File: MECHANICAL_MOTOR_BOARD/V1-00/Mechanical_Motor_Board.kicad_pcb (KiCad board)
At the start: 2 copper layers, 88.9 x 44.5 mm, 83 parts, among them K1 COLONETTE, K2 COLONETTE, K3 COLONETTE, K4 COLONETTE, P1001 CONN_02X13, P1002 CONN_02X08, P1003 CONN_01X02, P1004 CONN_01X02, P1005 CONN_01X04, P1006 CONN_01X04, Q2001 2N7002, Q3003 BSR14, Q3004 BSR14, Q3005 BTS50055, Q3006 BTS50055, Q3007 STB80NF55L_06T4, Q3008 STB80NF55L_06T4, Q3009 STB80NF55L_06T4, Q3010 STB80NF55L_06T4, Q3011 BTS50055, Q3012 BTS50055, Q3013 BSR14, Q3014 BSR14, U2001 HCTL-2032, U2002 M74VHC1GT02DTT1G, U3001 74HC02, U3002 74HC02, X2001 12Mhz

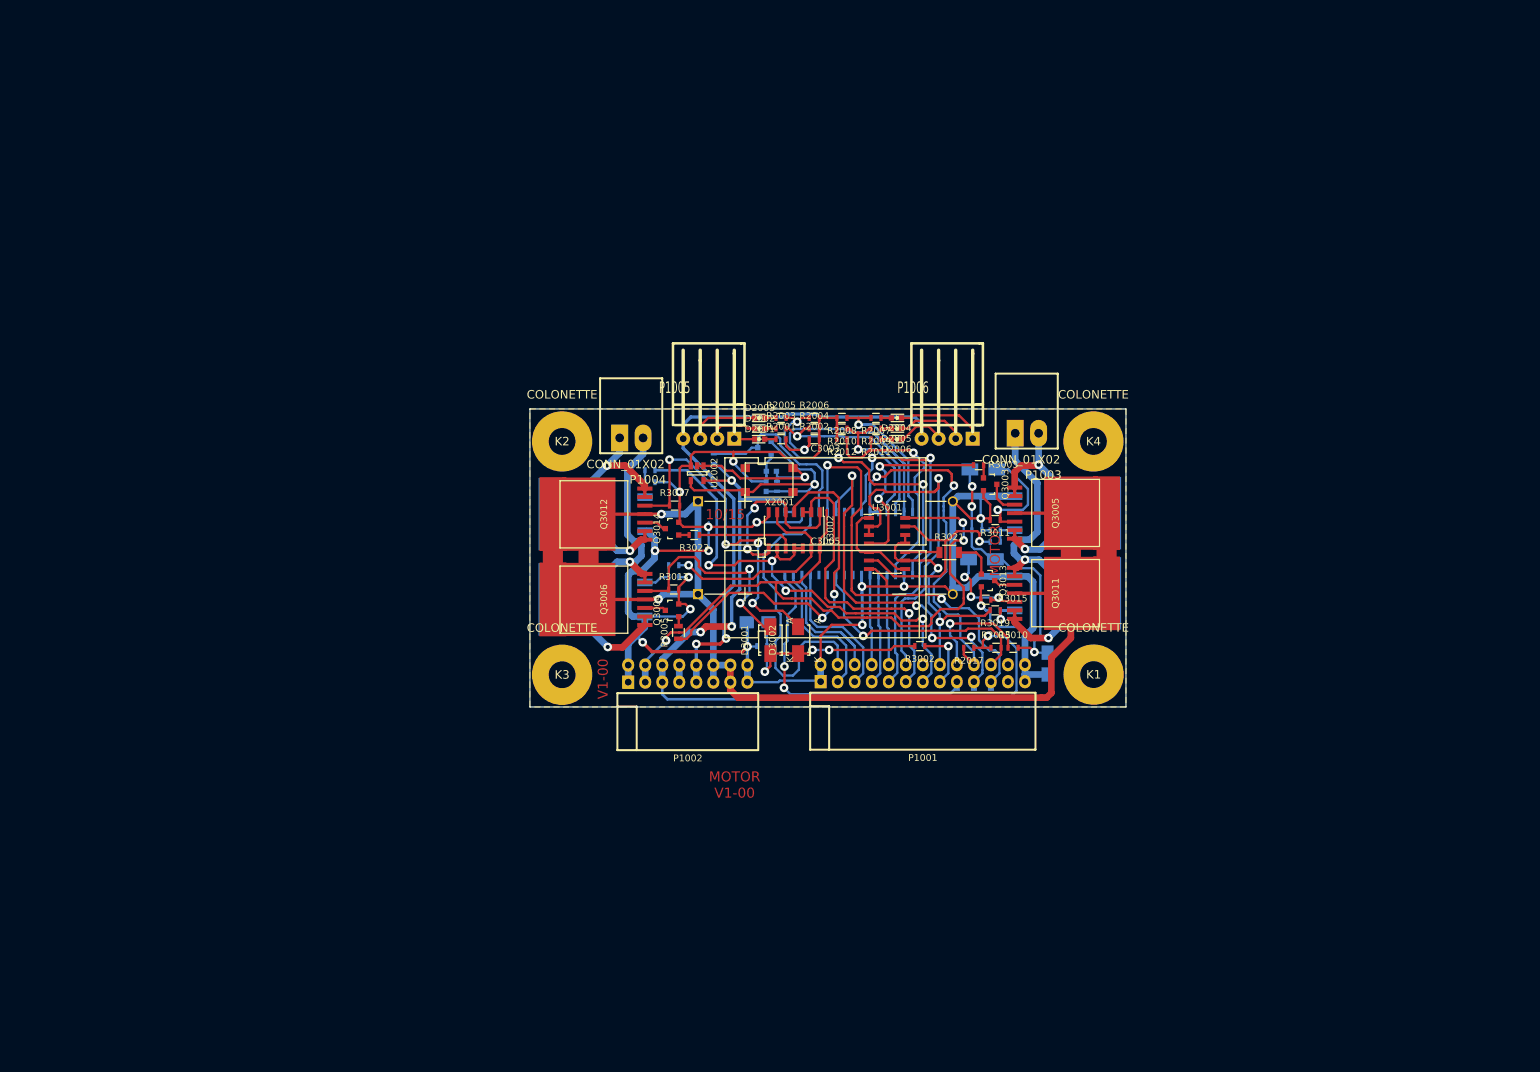
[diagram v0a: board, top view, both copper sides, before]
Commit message: MAJ 2018
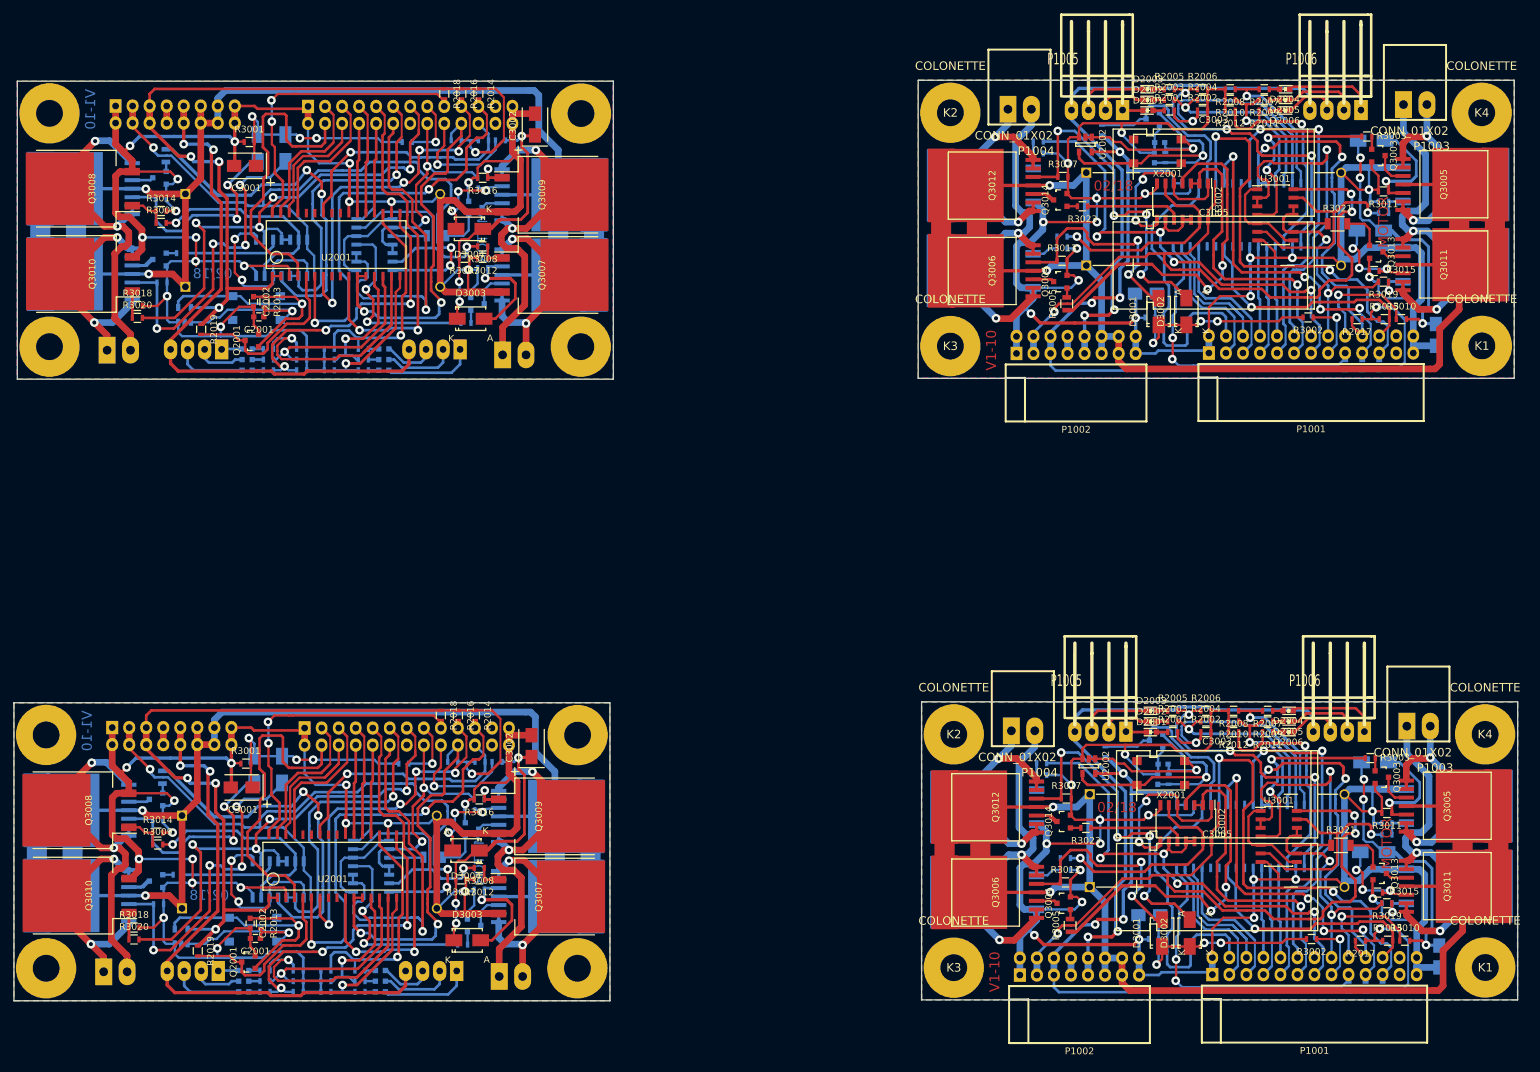
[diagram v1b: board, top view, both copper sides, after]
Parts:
- added C2001: 27p, Capacitors_SMD:C_0603, F.Cu at (73.3, 164.6)
- added C2001: 27p, Capacitors_SMD:C_0603, F.Cu at (73.8, 71.9)
- added C2001: 27p, Capacitors_SMD:C_0603, B.Cu at (208.7, 138.6)
- added C2002: 27p, Capacitors_SMD:C_0603, F.Cu at (72.5, 162.4)
- added C2002: 27p, Capacitors_SMD:C_0603, F.Cu at (73.0, 69.7)
- added C2002: 27p, Capacitors_SMD:C_0603, B.Cu at (207.9, 140.9)
- added C3001: 10u, Capacitors_Tantalum_SMD:TantalC_SizeB_EIA-3528_Wave, F.Cu at (71.2, 142.1)
- added C3001: 10u, Capacitors_Tantalum_SMD:TantalC_SizeB_EIA-3528_Wave, F.Cu at (71.8, 49.4)
- added C3001: 10u, Capacitors_Tantalum_SMD:TantalC_SizeB_EIA-3528_Wave, B.Cu at (206.6, 161.2)
- added C3002: 10u, Capacitors_Tantalum_SMD:TantalC_SizeB_EIA-3528_Wave, F.Cu at (114.5, 136.0)
- added C3002: 10u, Capacitors_Tantalum_SMD:TantalC_SizeB_EIA-3528_Wave, F.Cu at (115.0, 43.2)
- added C3002: 10u, Capacitors_Tantalum_SMD:TantalC_SizeB_EIA-3528_Wave, B.Cu at (249.9, 167.3)
- added C3003: 470U, Capacitors_ThroughHole:C_Axial_D13_L31_P38, B.Cu at (62.4, 160.1)
- added C3003: 470U, Capacitors_ThroughHole:C_Axial_D13_L31_P38, B.Cu at (62.9, 67.4)
- added C3003: 470U, Capacitors_ThroughHole:C_Axial_D13_L31_P38, F.Cu at (197.7, 143.1)
- added C3005: CP, Capacitors_ThroughHole:C_Axial_D13_L31_P38, B.Cu at (62.4, 146.3)
- added C3005: CP, Capacitors_ThroughHole:C_Axial_D13_L31_P38, B.Cu at (62.9, 53.6)
- added C3005: CP, Capacitors_ThroughHole:C_Axial_D13_L31_P38, F.Cu at (197.7, 157.0)
- added D2001: LED, LEDs:LED-0603, B.Cu at (71.6, 169.4)
- added D2001: LED, LEDs:LED-0603, B.Cu at (72.1, 76.7)
- added D2001: LED, LEDs:LED-0603, F.Cu at (206.9, 133.9)
- added D2002: LED, LEDs:LED-0603, B.Cu at (71.6, 171.0)
- added D2002: LED, LEDs:LED-0603, B.Cu at (72.1, 78.3)
- added D2002: LED, LEDs:LED-0603, F.Cu at (206.9, 132.3)
- added D2003: LED, LEDs:LED-0603, B.Cu at (71.6, 172.6)
- added D2003: LED, LEDs:LED-0603, B.Cu at (72.1, 79.9)
- added D2003: LED, LEDs:LED-0603, F.Cu at (206.9, 130.7)
- added D2004: LED, LEDs:LED-0603, B.Cu at (91.9, 172.6)
- added D2004: LED, LEDs:LED-0603, B.Cu at (92.5, 79.9)
- added D2004: LED, LEDs:LED-0603, F.Cu at (227.3, 130.7)
- added D2005: LED, LEDs:LED-0603, B.Cu at (91.9, 171.0)
- added D2005: LED, LEDs:LED-0603, B.Cu at (92.5, 78.3)
- added D2005: LED, LEDs:LED-0603, F.Cu at (227.3, 132.3)
- added D2006: LED, LEDs:LED-0603, B.Cu at (91.9, 169.4)
- added D2006: LED, LEDs:LED-0603, B.Cu at (92.5, 76.7)
- added D2006: LED, LEDs:LED-0603, F.Cu at (227.3, 133.9)
- added D3001: B140, Diodes_SMD:Diode-SMA_Standard, B.Cu at (73.2, 139.4)
- added D3001: B140, Diodes_SMD:Diode-SMA_Standard, B.Cu at (73.7, 46.7)
- added D3001: B140, Diodes_SMD:Diode-SMA_Standard, F.Cu at (208.5, 163.8)
- added D3002: B140, Diodes_SMD:Diode-SMA_Standard, B.Cu at (77.3, 139.4)
- added D3002: B140, Diodes_SMD:Diode-SMA_Standard, B.Cu at (77.8, 46.7)
- added D3002: B140, Diodes_SMD:Diode-SMA_Standard, F.Cu at (212.7, 163.8)
- added D3003: B140, Diodes_SMD:Diode-SMA_Standard, F.Cu at (104.9, 164.9)
- added D3003: B140, Diodes_SMD:Diode-SMA_Standard, F.Cu at (105.4, 72.2)
- added D3003: B140, Diodes_SMD:Diode-SMA_Standard, B.Cu at (240.3, 138.4)
- added D3004: B140, Diodes_SMD:Diode-SMA_Standard, F.Cu at (104.7, 151.5)
- added D3004: B140, Diodes_SMD:Diode-SMA_Standard, F.Cu at (105.2, 58.8)
- added D3004: B140, Diodes_SMD:Diode-SMA_Standard, B.Cu at (240.1, 151.8)
- added K1: COLONETTE, CEN-PCB:COLONETTE, B.Cu at (121.4, 134.3)
- added K1: COLONETTE, CEN-PCB:COLONETTE, B.Cu at (121.9, 41.6)
- added K1: COLONETTE, CEN-PCB:COLONETTE, F.Cu at (256.7, 169.0)
- added K2: COLONETTE, CEN-PCB:COLONETTE, B.Cu at (42.1, 169.1)
- added K2: COLONETTE, CEN-PCB:COLONETTE, B.Cu at (42.6, 76.4)
- added K2: COLONETTE, CEN-PCB:COLONETTE, F.Cu at (177.5, 134.2)
- added K3: COLONETTE, CEN-PCB:COLONETTE, B.Cu at (42.1, 134.3)
- added K3: COLONETTE, CEN-PCB:COLONETTE, B.Cu at (42.6, 41.6)
- added K3: COLONETTE, CEN-PCB:COLONETTE, F.Cu at (177.5, 169.0)
- added K4: COLONETTE, CEN-PCB:COLONETTE, B.Cu at (121.3, 169.1)
- added K4: COLONETTE, CEN-PCB:COLONETTE, B.Cu at (121.8, 76.4)
- added K4: COLONETTE, CEN-PCB:COLONETTE, F.Cu at (256.7, 134.2)
- added P1001: CONN_02X13, w_pin_strip:pin_socket_13x2-90, B.Cu at (95.9, 129.6)
- added P1001: CONN_02X13, w_pin_strip:pin_socket_13x2-90, B.Cu at (96.4, 36.9)
- added P1001: CONN_02X13, w_pin_strip:pin_socket_13x2-90, F.Cu at (231.3, 173.7)
- added P1002: CONN_02X08, w_pin_strip:pin_socket_8x2-90, B.Cu at (60.8, 129.5)
- added P1002: CONN_02X08, w_pin_strip:pin_socket_8x2-90, B.Cu at (61.3, 36.8)
- added P1002: CONN_02X08, w_pin_strip:pin_socket_8x2-90, F.Cu at (196.2, 173.7)
- added P1003: CONN_01X02, CEN-PCB:WEIDMULLER-SL-3.5-2-90G, B.Cu at (109.7, 170.3)
- added P1003: CONN_01X02, CEN-PCB:WEIDMULLER-SL-3.5-2-90G, B.Cu at (110.2, 77.6)
- added P1003: CONN_01X02, CEN-PCB:WEIDMULLER-SL-3.5-2-90G, F.Cu at (245.0, 133.0)
- added P1004: CONN_01X02, CEN-PCB:WEIDMULLER-SL-3.5-2-90G, B.Cu at (50.7, 169.6)
- added P1004: CONN_01X02, CEN-PCB:WEIDMULLER-SL-3.5-2-90G, B.Cu at (51.2, 76.9)
- added P1004: CONN_01X02, CEN-PCB:WEIDMULLER-SL-3.5-2-90G, F.Cu at (186.1, 133.7)
- added P1005: CONN_01X04, CEN-PCB:KK-4-H, B.Cu at (60.1, 169.5)
- added P1005: CONN_01X04, CEN-PCB:KK-4-H, B.Cu at (60.7, 76.8)
- added P1005: CONN_01X04, CEN-PCB:KK-4-H, F.Cu at (195.5, 133.8)
- added P1006: CONN_01X04, CEN-PCB:KK-4-H, B.Cu at (95.7, 169.5)
- added P1006: CONN_01X04, CEN-PCB:KK-4-H, B.Cu at (96.2, 76.8)
- added P1006: CONN_01X04, CEN-PCB:KK-4-H, F.Cu at (231.1, 133.8)
- added Q2001: 2N7002, Housings_SOT-23_SOT-143_TSOT-6:SOT-23, F.Cu at (72.3, 168.1)
- added Q2001: 2N7002, Housings_SOT-23_SOT-143_TSOT-6:SOT-23, F.Cu at (72.8, 75.4)
- added Q2001: 2N7002, Housings_SOT-23_SOT-143_TSOT-6:SOT-23, B.Cu at (207.6, 135.1)
- added Q3003: BSR14, Housings_SOT-23_SOT-143_TSOT-6:SOT-23, B.Cu at (105.9, 162.7)
- added Q3003: BSR14, Housings_SOT-23_SOT-143_TSOT-6:SOT-23, B.Cu at (106.4, 70.0)
- added Q3003: BSR14, Housings_SOT-23_SOT-143_TSOT-6:SOT-23, F.Cu at (241.3, 140.6)
- added Q3004: BSR14, Housings_SOT-23_SOT-143_TSOT-6:SOT-23, B.Cu at (58.5, 143.9)
- added Q3004: BSR14, Housings_SOT-23_SOT-143_TSOT-6:SOT-23, B.Cu at (59.0, 51.2)
- added Q3004: BSR14, Housings_SOT-23_SOT-143_TSOT-6:SOT-23, F.Cu at (193.9, 159.4)
- added Q3005: BTS50055, f4deb-mod-library:PG-TO220-7-4, B.Cu at (109.6, 158.4)
- added Q3005: BTS50055, f4deb-mod-library:PG-TO220-7-4, B.Cu at (110.1, 65.7)
- added Q3005: BTS50055, f4deb-mod-library:PG-TO220-7-4, F.Cu at (245.0, 144.9)
- added Q3006: BTS50055, f4deb-mod-library:PG-TO220-7-4, B.Cu at (54.4, 145.5)
- added Q3006: BTS50055, f4deb-mod-library:PG-TO220-7-4, B.Cu at (54.9, 52.8)
- added Q3006: BTS50055, f4deb-mod-library:PG-TO220-7-4, F.Cu at (189.8, 157.8)
- added Q3007: STB80NF55L_06T4, SMD_Packages:TO-263, F.Cu at (109.6, 158.4)
- added Q3007: STB80NF55L_06T4, SMD_Packages:TO-263, F.Cu at (110.1, 65.7)
- added Q3007: STB80NF55L_06T4, SMD_Packages:TO-263, B.Cu at (245.0, 144.9)
- added Q3008: STB80NF55L_06T4, SMD_Packages:TO-263, F.Cu at (54.4, 145.5)
- added Q3008: STB80NF55L_06T4, SMD_Packages:TO-263, F.Cu at (54.9, 52.8)
- added Q3008: STB80NF55L_06T4, SMD_Packages:TO-263, B.Cu at (189.8, 157.8)
- added Q3009: STB80NF55L_06T4, SMD_Packages:TO-263, F.Cu at (109.6, 146.4)
- added Q3009: STB80NF55L_06T4, SMD_Packages:TO-263, F.Cu at (110.1, 53.7)
- added Q3009: STB80NF55L_06T4, SMD_Packages:TO-263, B.Cu at (245.0, 156.9)
- added Q3010: STB80NF55L_06T4, SMD_Packages:TO-263, F.Cu at (54.4, 158.2)
- added Q3010: STB80NF55L_06T4, SMD_Packages:TO-263, F.Cu at (55.0, 65.5)
- added Q3010: STB80NF55L_06T4, SMD_Packages:TO-263, B.Cu at (189.8, 145.0)
- added Q3011: BTS50055, f4deb-mod-library:PG-TO220-7-4, B.Cu at (109.6, 146.4)
- added Q3011: BTS50055, f4deb-mod-library:PG-TO220-7-4, B.Cu at (110.1, 53.7)
- added Q3011: BTS50055, f4deb-mod-library:PG-TO220-7-4, F.Cu at (245.0, 156.9)
- added Q3012: BTS50055, f4deb-mod-library:PG-TO220-7-4, B.Cu at (54.4, 158.2)
- added Q3012: BTS50055, f4deb-mod-library:PG-TO220-7-4, B.Cu at (54.9, 65.5)
- added Q3012: BTS50055, f4deb-mod-library:PG-TO220-7-4, F.Cu at (189.8, 145.0)
- added Q3013: BSR14, Housings_SOT-23_SOT-143_TSOT-6:SOT-23, B.Cu at (105.6, 148.3)
- added Q3013: BSR14, Housings_SOT-23_SOT-143_TSOT-6:SOT-23, B.Cu at (106.1, 55.6)
- added Q3013: BSR14, Housings_SOT-23_SOT-143_TSOT-6:SOT-23, F.Cu at (241.0, 154.9)
- added Q3014: BSR14, Housings_SOT-23_SOT-143_TSOT-6:SOT-23, B.Cu at (58.5, 156.1)
- added Q3014: BSR14, Housings_SOT-23_SOT-143_TSOT-6:SOT-23, B.Cu at (59.0, 63.4)
- added Q3014: BSR14, Housings_SOT-23_SOT-143_TSOT-6:SOT-23, F.Cu at (193.9, 147.2)
- added R2001: 2.1k, Resistors_SMD:R_0603, B.Cu at (74.7, 169.4)
- added R2001: 2.1k, Resistors_SMD:R_0603, B.Cu at (75.2, 76.7)
- added R2001: 2.1k, Resistors_SMD:R_0603, F.Cu at (210.1, 133.9)
- added R2002: 2.1k, Resistors_SMD:R_0603, B.Cu at (79.7, 169.4)
- added R2002: 2.1k, Resistors_SMD:R_0603, B.Cu at (80.2, 76.7)
- added R2002: 2.1k, Resistors_SMD:R_0603, F.Cu at (215.1, 133.9)
- added R2003: 2.1k, Resistors_SMD:R_0603, B.Cu at (74.7, 171.0)
- added R2003: 2.1k, Resistors_SMD:R_0603, B.Cu at (75.2, 78.3)
- added R2003: 2.1k, Resistors_SMD:R_0603, F.Cu at (210.1, 132.3)
- added R2004: 2.1k, Resistors_SMD:R_0603, B.Cu at (79.7, 171.0)
- added R2004: 2.1k, Resistors_SMD:R_0603, B.Cu at (80.2, 78.3)
- added R2004: 2.1k, Resistors_SMD:R_0603, F.Cu at (215.1, 132.3)
- added R2005: 2.1k, Resistors_SMD:R_0603, B.Cu at (74.7, 172.6)
- added R2005: 2.1k, Resistors_SMD:R_0603, B.Cu at (75.2, 79.9)
- added R2005: 2.1k, Resistors_SMD:R_0603, F.Cu at (210.1, 130.7)
- added R2006: 2.1k, Resistors_SMD:R_0603, B.Cu at (79.7, 172.6)
- added R2006: 2.1k, Resistors_SMD:R_0603, B.Cu at (80.2, 79.9)
- added R2006: 2.1k, Resistors_SMD:R_0603, F.Cu at (215.1, 130.7)
- added R2007: 2.1k, Resistors_SMD:R_0603, B.Cu at (88.9, 172.6)
- added R2007: 2.1k, Resistors_SMD:R_0603, B.Cu at (89.4, 79.9)
- added R2007: 2.1k, Resistors_SMD:R_0603, F.Cu at (224.3, 130.7)
- added R2008: 2.1k, Resistors_SMD:R_0603, B.Cu at (83.8, 172.6)
- added R2008: 2.1k, Resistors_SMD:R_0603, B.Cu at (84.3, 79.9)
- added R2008: 2.1k, Resistors_SMD:R_0603, F.Cu at (219.2, 130.7)
- added R2009: 2.1k, Resistors_SMD:R_0603, B.Cu at (88.9, 171.0)
- added R2009: 2.1k, Resistors_SMD:R_0603, B.Cu at (89.4, 78.3)
- added R2009: 2.1k, Resistors_SMD:R_0603, F.Cu at (224.3, 132.3)
- added R2010: 2.1k, Resistors_SMD:R_0603, B.Cu at (83.8, 171.0)
- added R2010: 2.1k, Resistors_SMD:R_0603, B.Cu at (84.3, 78.3)
- added R2010: 2.1k, Resistors_SMD:R_0603, F.Cu at (219.2, 132.3)
- added R2011: 2.1k, Resistors_SMD:R_0603, B.Cu at (88.9, 169.4)
- added R2011: 2.1k, Resistors_SMD:R_0603, B.Cu at (89.4, 76.7)
- added R2011: 2.1k, Resistors_SMD:R_0603, F.Cu at (224.3, 133.9)
- added R2012: 2.1k, Resistors_SMD:R_0603, B.Cu at (83.8, 169.4)
- added R2012: 2.1k, Resistors_SMD:R_0603, B.Cu at (84.3, 76.7)
- added R2012: 2.1k, Resistors_SMD:R_0603, F.Cu at (219.2, 133.9)
- added R2013: 10M, Resistors_SMD:R_0603, F.Cu at (74.1, 162.4)
- added R2013: 10M, Resistors_SMD:R_0603, F.Cu at (74.6, 69.7)
- added R2013: 10M, Resistors_SMD:R_0603, B.Cu at (209.5, 140.9)
- added R2014: 10k, Resistors_SMD:R_0603, F.Cu at (106.0, 131.4)
- added R2014: 10k, Resistors_SMD:R_0603, F.Cu at (106.6, 38.7)
- added R2014: 10k, Resistors_SMD:R_0603, B.Cu at (241.4, 171.9)
- added R2015: 10k, Resistors_SMD:R_0603, B.Cu at (106.8, 138.3)
- added R2015: 10k, Resistors_SMD:R_0603, B.Cu at (107.3, 45.6)
- added R2015: 10k, Resistors_SMD:R_0603, F.Cu at (242.2, 165.0)
- added R2016: 10k, Resistors_SMD:R_0603, F.Cu at (103.5, 131.4)
- added R2016: 10k, Resistors_SMD:R_0603, F.Cu at (104.0, 38.7)
- added R2016: 10k, Resistors_SMD:R_0603, B.Cu at (238.9, 171.9)
- added R2017: 10k, Resistors_SMD:R_0603, B.Cu at (102.7, 138.3)
- added R2017: 10k, Resistors_SMD:R_0603, B.Cu at (103.3, 45.6)
- added R2017: 10k, Resistors_SMD:R_0603, F.Cu at (238.1, 165.0)
- added R2018: 10k, Resistors_SMD:R_0603, F.Cu at (101.0, 131.4)
- added R2018: 10k, Resistors_SMD:R_0603, F.Cu at (101.5, 38.7)
- added R2018: 10k, Resistors_SMD:R_0603, B.Cu at (236.3, 171.9)
- added R2019: 1k, Resistors_SMD:R_0603, F.Cu at (64.7, 166.5)
- added R2019: 1k, Resistors_SMD:R_0603, F.Cu at (65.2, 73.8)
- added R2019: 1k, Resistors_SMD:R_0603, B.Cu at (200.1, 136.8)
- added R3001: 100k, Resistors_SMD:R_0603, F.Cu at (71.9, 138.6)
- added R3001: 100k, Resistors_SMD:R_0603, F.Cu at (72.4, 45.8)
- added R3001: 100k, Resistors_SMD:R_0603, B.Cu at (207.3, 164.7)
- added R3002: 10k, Resistors_SMD:R_0603, B.Cu at (95.4, 138.6)
- added R3002: 10k, Resistors_SMD:R_0603, B.Cu at (95.9, 45.8)
- added R3002: 10k, Resistors_SMD:R_0603, F.Cu at (230.8, 164.7)
- added R3003: 10k, Resistors_SMD:R_0603, B.Cu at (104.2, 165.5)
- added R3003: 10k, Resistors_SMD:R_0603, B.Cu at (104.7, 72.8)
- added R3003: 10k, Resistors_SMD:R_0603, F.Cu at (239.6, 137.7)
- added R3005: 10k, Resistors_SMD:R_0805, B.Cu at (59.4, 140.6)
- added R3005: 10k, Resistors_SMD:R_0805, B.Cu at (59.9, 47.9)
- added R3005: 10k, Resistors_SMD:R_0805, F.Cu at (194.8, 162.7)
- added R3007: 100k, Resistors_SMD:R_0603, F.Cu at (103.9, 155.8)
- added R3007: 100k, Resistors_SMD:R_0603, F.Cu at (104.5, 63.1)
- added R3007: 100k, Resistors_SMD:R_0603, B.Cu at (239.3, 147.4)
- added R3008: 100, Resistors_SMD:R_0603, F.Cu at (106.7, 154.1)
- added R3008: 100, Resistors_SMD:R_0603, F.Cu at (107.2, 61.4)
- added R3008: 100, Resistors_SMD:R_0603, B.Cu at (242.1, 149.2)
- added R3009: 100, Resistors_SMD:R_0603, F.Cu at (58.7, 150.6)
- added R3009: 100, Resistors_SMD:R_0603, F.Cu at (59.2, 57.9)
- added R3009: 100, Resistors_SMD:R_0603, B.Cu at (194.1, 152.7)
- added R3010: 10k, Resistors_SMD:R_0603, B.Cu at (109.3, 138.3)
- added R3010: 10k, Resistors_SMD:R_0603, B.Cu at (109.9, 45.6)
- added R3010: 10k, Resistors_SMD:R_0603, F.Cu at (244.7, 165.0)
- added R3011: 2.2k, Resistors_SMD:R_0603, B.Cu at (106.7, 157.4)
- added R3011: 2.2k, Resistors_SMD:R_0603, B.Cu at (107.2, 64.6)
- added R3011: 2.2k, Resistors_SMD:R_0603, F.Cu at (242.1, 145.9)
- added R3012: 100k, Resistors_SMD:R_0603, F.Cu at (106.7, 155.8)
- added R3012: 100k, Resistors_SMD:R_0603, F.Cu at (107.2, 63.1)
- added R3012: 100k, Resistors_SMD:R_0603, B.Cu at (242.1, 147.4)
- added R3013: 2.2k, Resistors_SMD:R_0603, B.Cu at (58.7, 147.0)
- added R3013: 2.2k, Resistors_SMD:R_0603, B.Cu at (59.2, 54.3)
- added R3013: 2.2k, Resistors_SMD:R_0603, F.Cu at (194.1, 156.3)
- added R3014: 100k, Resistors_SMD:R_0603, F.Cu at (58.7, 148.8)
- added R3014: 100k, Resistors_SMD:R_0603, F.Cu at (59.2, 56.1)
- added R3014: 100k, Resistors_SMD:R_0603, B.Cu at (194.1, 154.4)
- added R3015: 2.2k, Resistors_SMD:R_0603, B.Cu at (105.3, 145.5)
- added R3015: 2.2k, Resistors_SMD:R_0603, B.Cu at (105.8, 52.8)
- added R3015: 2.2k, Resistors_SMD:R_0603, F.Cu at (240.7, 157.8)
- added R3016: 100k, Resistors_SMD:R_0603, F.Cu at (106.7, 143.9)
- added R3016: 100k, Resistors_SMD:R_0603, F.Cu at (107.2, 51.2)
- added R3016: 100k, Resistors_SMD:R_0603, B.Cu at (242.1, 159.4)
- added R3017: 2.2k, Resistors_SMD:R_0603, B.Cu at (58.9, 159.5)
- added R3017: 2.2k, Resistors_SMD:R_0603, B.Cu at (59.4, 66.8)
- added R3017: 2.2k, Resistors_SMD:R_0603, F.Cu at (194.2, 143.8)
- added R3018: 100k, Resistors_SMD:R_0603, F.Cu at (55.2, 163.0)
- added R3018: 100k, Resistors_SMD:R_0603, F.Cu at (55.7, 70.3)
- added R3018: 100k, Resistors_SMD:R_0603, B.Cu at (190.6, 140.3)
- added R3019: 100, Resistors_SMD:R_0603, B.Cu at (106.7, 143.9)
- added R3019: 100, Resistors_SMD:R_0603, B.Cu at (107.2, 51.2)
- added R3019: 100, Resistors_SMD:R_0603, F.Cu at (242.1, 159.4)
- added R3020: 100, Resistors_SMD:R_0603, F.Cu at (55.2, 164.8)
- added R3020: 100, Resistors_SMD:R_0603, F.Cu at (55.7, 72.1)
- added R3020: 100, Resistors_SMD:R_0603, B.Cu at (190.6, 138.5)
- added R3021: 10k, Resistors_SMD:R_1206, B.Cu at (99.8, 152.5)
- added R3021: 10k, Resistors_SMD:R_1206, B.Cu at (100.3, 59.8)
- added R3021: 10k, Resistors_SMD:R_1206, F.Cu at (235.2, 150.7)
- added R3023: 10k, Resistors_SMD:R_0603, B.Cu at (61.8, 155.1)
- added R3023: 10k, Resistors_SMD:R_0603, B.Cu at (62.3, 62.4)
- added R3023: 10k, Resistors_SMD:R_0603, F.Cu at (197.2, 148.1)
- added U2001: HCTL-2032, SMD_Packages:SOJ-32, F.Cu at (84.8, 153.9)
- added U2001: HCTL-2032, SMD_Packages:SOJ-32, F.Cu at (85.3, 61.2)
- added U2001: HCTL-2032, SMD_Packages:SOJ-32, B.Cu at (220.2, 149.4)
- added U2002: M74VHC1GT02DTT1G, Housings_SOT-23_SOT-143_TSOT-6:SOT-23-5, B.Cu at (62.2, 164.3)
- added U2002: M74VHC1GT02DTT1G, Housings_SOT-23_SOT-143_TSOT-6:SOT-23-5, B.Cu at (62.7, 71.6)
- added U2002: M74VHC1GT02DTT1G, Housings_SOT-23_SOT-143_TSOT-6:SOT-23-5, F.Cu at (197.6, 138.9)
- added U3001: 74HC02, Housings_SOIC:SOIC-14_3.9x8.7mm_Pitch1.27mm, B.Cu at (90.6, 153.9)
- added U3001: 74HC02, Housings_SOIC:SOIC-14_3.9x8.7mm_Pitch1.27mm, B.Cu at (91.1, 61.2)
- added U3001: 74HC02, Housings_SOIC:SOIC-14_3.9x8.7mm_Pitch1.27mm, F.Cu at (225.9, 149.4)
- added U3002: 74HC02, Housings_SOIC:SOIC-14_3.9x8.7mm_Pitch1.27mm, B.Cu at (76.7, 155.8)
- added U3002: 74HC02, Housings_SOIC:SOIC-14_3.9x8.7mm_Pitch1.27mm, B.Cu at (77.2, 63.1)
- added U3002: 74HC02, Housings_SOIC:SOIC-14_3.9x8.7mm_Pitch1.27mm, F.Cu at (212.1, 147.4)
- added X2001: 12Mhz, f4deb-mod-library:MDX75104, B.Cu at (73.0, 163.3)
- added X2001: 12Mhz, f4deb-mod-library:MDX75104, B.Cu at (73.5, 70.6)
- added X2001: 12Mhz, f4deb-mod-library:MDX75104, F.Cu at (208.3, 140.0)
- moved C2001 75.9 mm to (208.2, 45.9)
- moved C3002 75.9 mm to (249.4, 74.6)
- moved C3003 75.9 mm to (197.2, 50.4)
- moved C3005 75.9 mm to (197.2, 64.3)
- moved D2003 75.9 mm to (206.4, 38.0)
- moved D2004 75.9 mm to (226.8, 38.0)
- moved K1 75.9 mm to (256.2, 76.3)
- moved P1002 75.9 mm to (195.7, 81.0)
- moved P1003 75.9 mm to (244.5, 40.3)
- moved P1005 75.9 mm to (195.0, 41.1)
- moved P1006 75.9 mm to (230.6, 41.1)
- moved Q3006 75.9 mm to (189.3, 65.1)
- moved Q3008 75.9 mm to (189.3, 65.1)
- moved R2007 75.9 mm to (223.8, 38.0)
- moved R2014 75.9 mm to (240.9, 79.2)
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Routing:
- net GND: track 322.6 -> 1292.9 mm, vias 15 -> 60
- net +15V: track 220.2 -> 880.7 mm, vias 2 -> 8
- net +5VD: track 132.1 -> 570.5 mm, vias 4 -> 16
- net +3V3: track 101.9 -> 407.7 mm, vias 3 -> 12
- net +12V: track 88.2 -> 352.9 mm, vias 2 -> 8
- net /Motor/IO9: track 76.7 -> 315.9 mm, vias 4 -> 16
- net Net-(C3002-Pad1): track 40.3 -> 250.9 mm, vias 3 -> 12
- net /Codeur/IO1: track 64.4 -> 257.6 mm, vias 2 -> 8
- net /Codeur/IO4: track 60.4 -> 247.5 mm, vias 2 -> 8
- net /Motor/M1B: track 61.9 -> 247.7 mm, vias 2 -> 8
- net /Codeur/IO25: track 56.6 -> 219.9 mm, vias 2 -> 8
- net /Motor/M2A: track 54.4 -> 217.7 mm, vias 2 -> 8
- net /Codeur/IO3: track 57.3 -> 220.5 mm, vias 4 -> 16
- net /Motor/OC5-5V: track 54.0 -> 216.1 mm, vias 1 -> 4
- net Net-(R3005-Pad1): track 53.8 -> 214.1 mm, vias 2 -> 8
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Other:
- board size 88.9 x 44.5 mm -> 224.3 x 137.3 mm
- board text added: "02/18"
- board text added: "V1-10"
- board text removed: "10/15"
- board text removed: "MOTOR V1-00"
- board text removed: "V1-00"
